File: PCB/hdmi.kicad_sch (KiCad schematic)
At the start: 25 parts, among them J3 HDMI-019S, U12 PCA9306DC1, U14 UCL0524P, U15 UCL0524P, U16 UCL0524P

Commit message: cleaning up USB-C, switching some of the decoupling and assigning a bunch of footprints
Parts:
- C121: footprint (none) -> Capacitor_SMD:C_0402_1005Metric
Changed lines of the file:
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@@
 			)
 		)
-		(property "Footprint" ""
+		(property "Footprint" "Capacitor_SMD:C_0402_1005Metric"
 			(at 147.0152 74.93 0)
 			(effects

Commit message: finished add in all the footprints
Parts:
- J3: footprint (none) -> Connector_Video:HDMI_A_Molex_208658-1001_Horizontal
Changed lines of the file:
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@@
 			)
 		)
-		(property "Footprint" ""
+		(property "Footprint" "Connector_Video:HDMI_A_Molex_208658-1001_Horizontal"
 			(at 126.365 107.95 0)
 			(effects

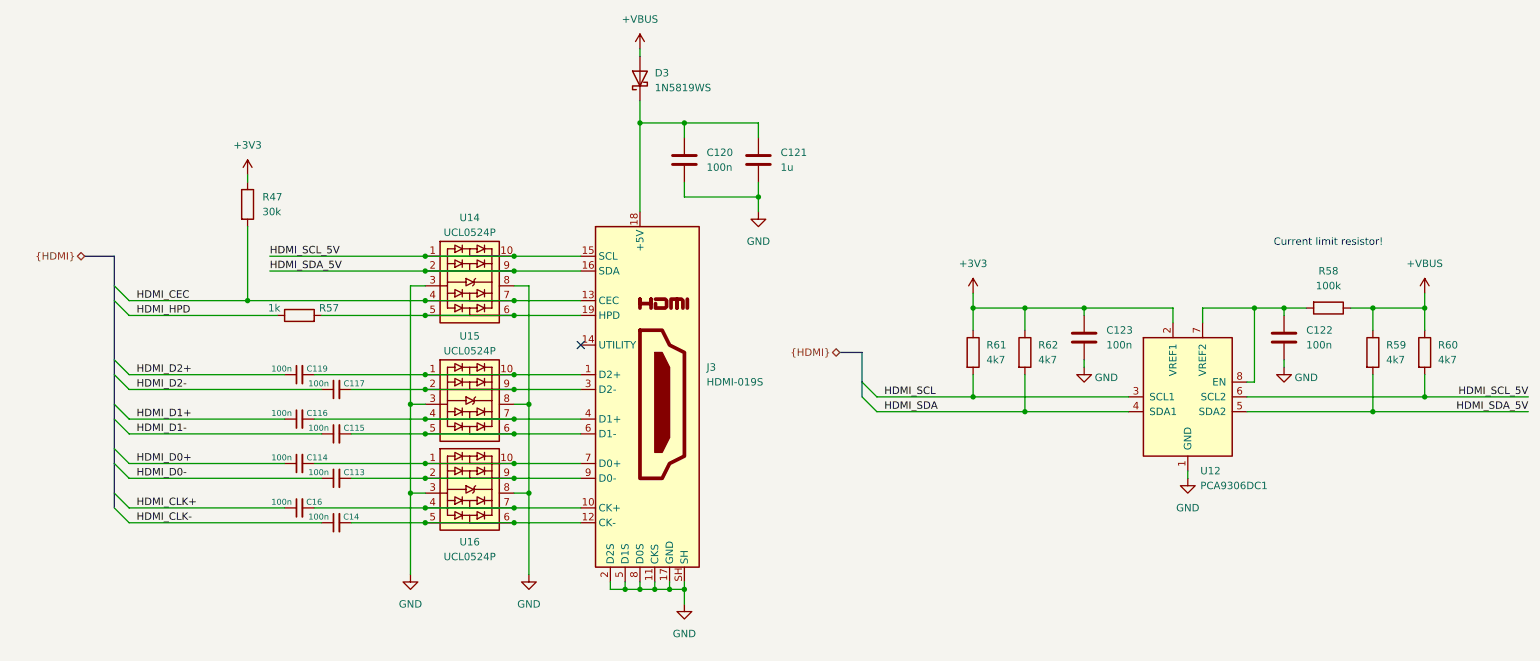
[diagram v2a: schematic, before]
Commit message: replacing the HDMI connector with micro HDMI
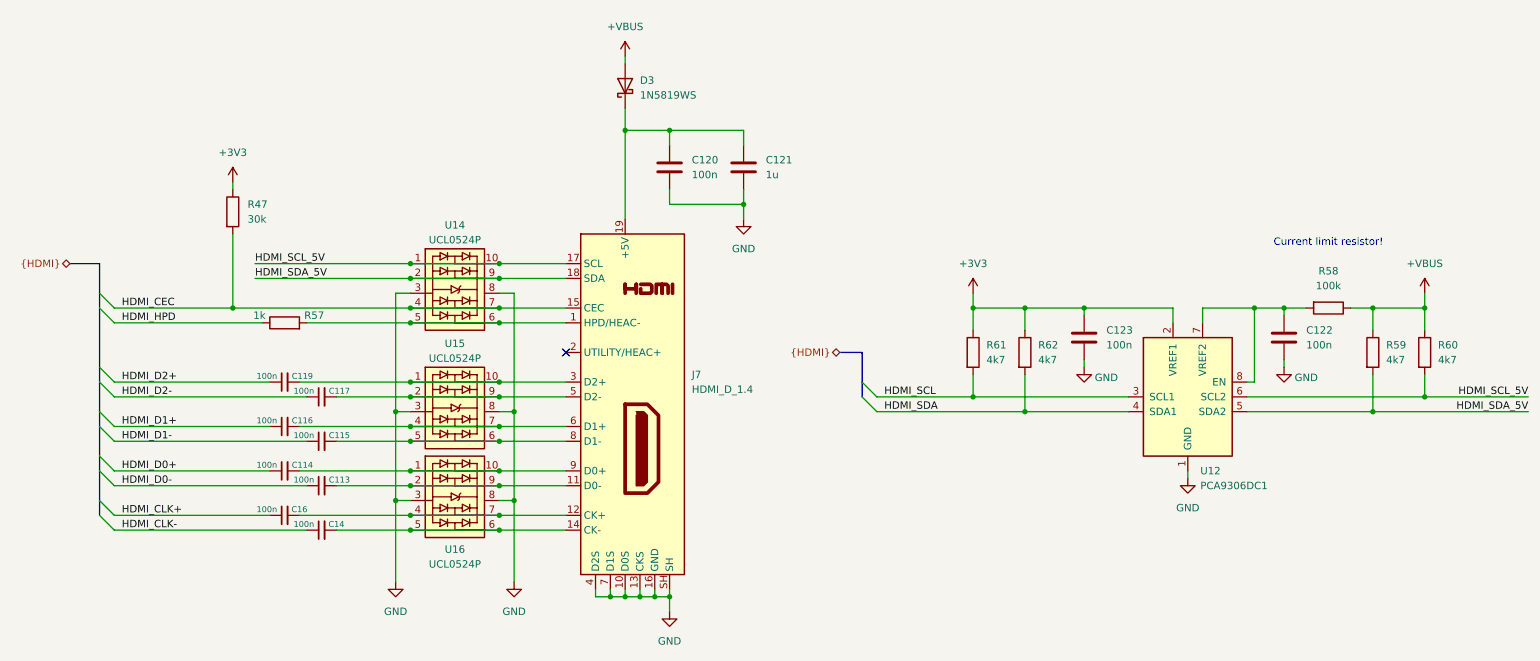
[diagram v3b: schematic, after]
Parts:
- removed J3: HDMI-019S, Connector_Video:HDMI_A_Molex_208658-1001_Horizontal, symbol FPGA Accelerator:HDMI_A
- added J7: HDMI_D_1.4, Connector_Video:HDMI_Micro-D_Molex_46765-1xxx, symbol FPGA Accelerator:HDMI_D_1.4
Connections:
- net GND: now also J7.10 (D0S), J7.13 (CKS), J7.16 (GND), J7.4 (D2S), J7.7 (D1S), J7.SH
- net HDMI_CEC: now also J7.15 (CEC)
- net HDMI_SCL_5V: now also J7.17 (SCL)
- net HDMI_SDA_5V: now also J7.18 (SDA)
- net at R57.2, U14.5, U14.6: now also J7.1 (HPD/HEAC-)
- net at C117.2, U15.2, U15.9: now also J7.5 (D2-)
- net at C120.1, C121.1, D3.1 (K): now also J7.19 (+5V)
- net at C116.2, U15.4, U15.7: now also J7.6 (D1+)
- net at C114.2, U16.1, U16.10: now also J7.9 (D0+)
- net at C119.2, U15.1, U15.10: now also J7.3 (D2+)
- net at C16.2, U16.4, U16.7: now also J7.12 (CK+)
- net at C14.2, U16.5, U16.6: now also J7.14 (CK-)
- net at C115.2, U15.5, U15.6: now also J7.8 (D1-)
- net at C113.2, U16.2, U16.9: now also J7.11 (D0-)
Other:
- moved on the sheet: C113, C114, C115, C116, C117, C119, C120, C121, C14, C16, D3, R47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

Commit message: adding some MPN's in, searching for ethernet RJ45's
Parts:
- J7: LCSC (none) -> C711358; MPN (none) -> HYC23-HDMID19-650
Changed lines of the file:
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@@
+			)
+		)
+		(property "MPN" "HYC23-HDMID19-650"
+			(at 123.19 109.22 0)
+			(effects
+				(font
+					(size 1.27 1.27)
+				)
+				(hide yes)
+			)
+		)
+		(property "LCSC" "C711358"
+			(at 123.19 109.22 0)
+			(effects
+				(font
+					(size 1.27 1.27)
+				)
+				(hide yes)
 			)
 		)
